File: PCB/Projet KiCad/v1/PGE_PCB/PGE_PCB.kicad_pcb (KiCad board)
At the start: 2 copper layers, 77 x 61.5 mm, 50 parts, among them CN2 Conn_01x02, J1 Conn_01x03, P1 USB_C_Plug_USB2.0, SW1 SW_Push, U1 STM32L476RGTx, U2 MCP73831T, U3 DS2438AZ+, U4 LD39050PU33R, U5 SiP32431DR3, Y1 ABS25-32.768KHZ-T

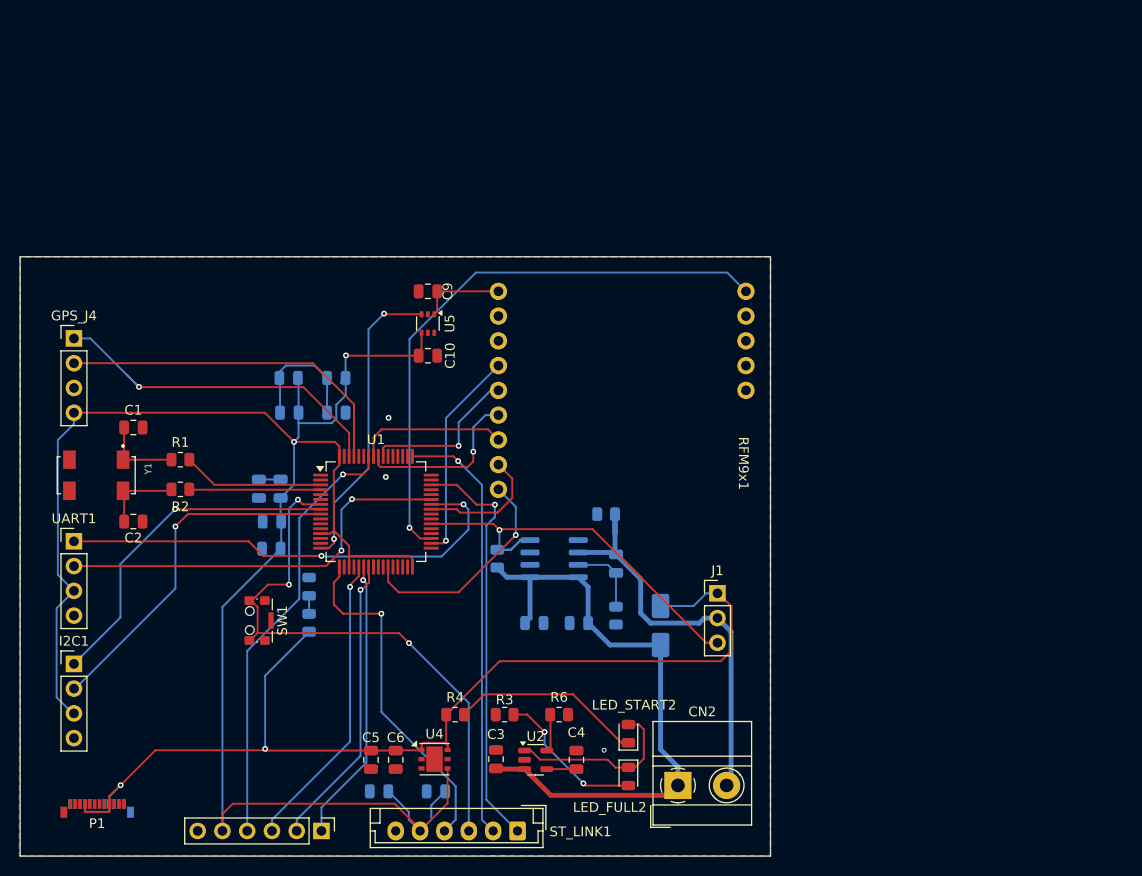
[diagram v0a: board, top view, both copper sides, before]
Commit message: Pcb VERSION GPS séparer
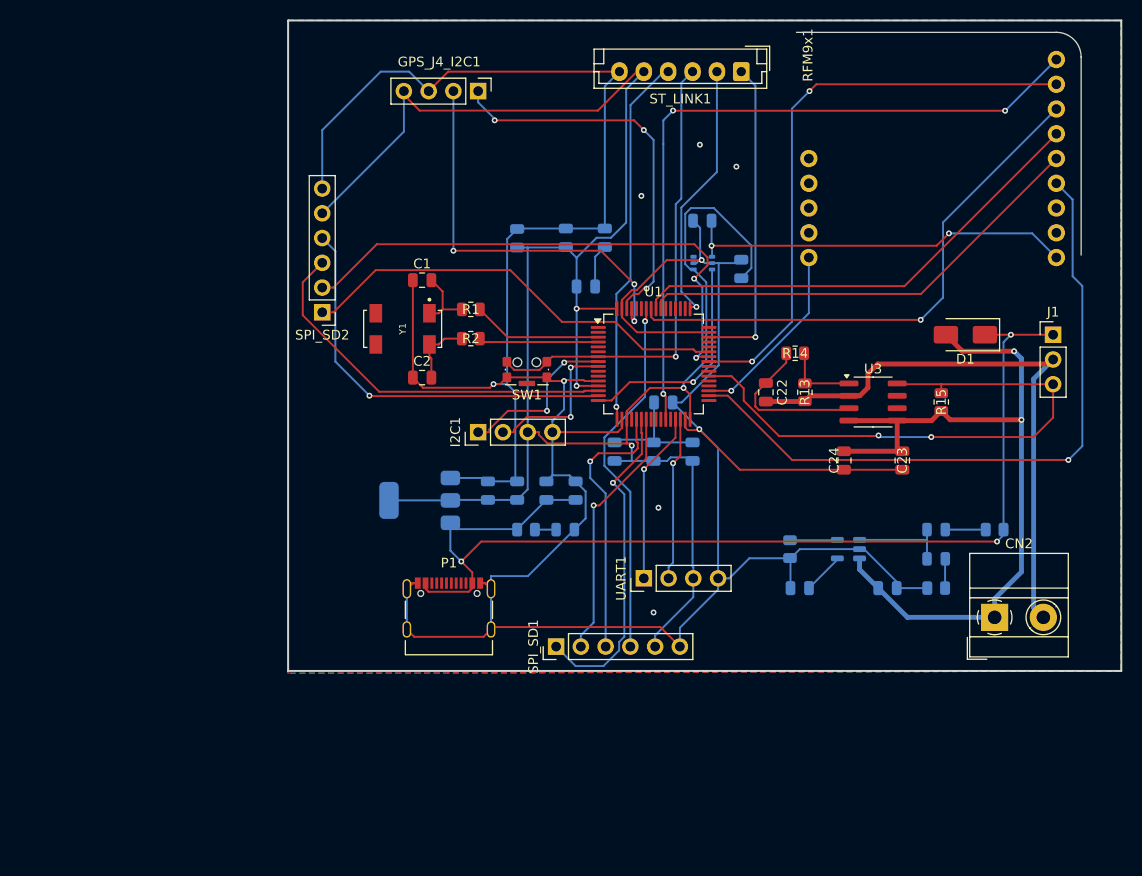
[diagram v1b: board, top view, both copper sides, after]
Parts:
- removed GPS_J4: Conn_01x04_Pin, Connector_PinHeader_2.54mm:PinHeader_1x04_P2.54mm_Vertical
- removed U4: LD39050PU33R, Package_DFN_QFN:DFN-6-1EP_3x3mm_P0.95mm_EP1.7x2.6mm
- added GPS_J4_I2C1: Conn_01x04_Pin, Connector_PinHeader_2.54mm:PinHeader_1x04_P2.54mm_Vertical, F.Cu at (138.0, 46.0)
- added SPI_SD2: Conn_01x06_Socket, Connector_PinHeader_2.54mm:PinHeader_1x06_P2.54mm_Vertical, F.Cu at (122.0, 68.7)
- added U6: LD1117S33TR_SOT223, Package_TO_SOT_SMD:SOT-223-3_TabPin2, B.Cu at (132.0, 88.0)
- C10, C3, C4, C5, C6, C9, LED_FULL2, LED_START2, R3, R4, R6, U2, U5: moved to B.Cu
- C22, C23, C24, D1, R13, R14, R15, U3: moved to F.Cu
- P1: footprint Connector_USB:USB_C_Plug_Molex_105444 -> Connector_USB:USB_C_Receptacle_Palconn_UTC16-G
- moved ST_LINK1 81.2 mm to (165.0, 44.0)
- moved UART1 58.6 mm to (155.0, 96.0), turned to 90 degrees
- moved R4 58.5 mm to (191.0, 91.0), turned to 0 degrees
- moved R15 48.3 mm to (185.5, 77.9)
- moved I2C1 47.8 mm to (138.0, 81.0), turned to 90 degrees
- moved R3 46.1 mm to (185.0, 97.0)
- moved C19 44.0 mm to (147.0, 61.0), turned to 90 degrees
- moved C18 43.9 mm to (151.0, 61.0), turned to 90 degrees
- moved C3 43.8 mm to (180.0, 97.0), turned to 180 degrees
- moved J1 43.5 mm to (197.0, 71.0)
- moved D1 43.2 mm to (188.0, 71.0), turned to 180 degrees
- moved C14 42.1 mm to (160.0, 83.0), turned to 90 degrees
- moved P1 41.3 mm to (135.0, 99.0)
- moved RFM9x1 39.1 mm to (184.0, 52.7), turned to 90 degrees
- moved U2 38.7 mm to (176.0, 93.0), turned to 180 degrees
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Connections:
- U1 pad 14: unconnected-(U1-PA0-Pad14) -> standby
- U1 pad 15: unconnected-(U1-PA1-Pad15) -> GPS_reset
- U1 pad 29: unconnected-(U1-PB10-Pad29) -> Tx_uart
- U1 pad 30: unconnected-(U1-PB11-Pad30) -> Rx_uart
- U1 pad 42: Tx_uart -> GPS_RX
- U1 pad 43: Rx_uart -> GPS_TX
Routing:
- net VREF-: track 0.00 -> 348.6 mm, vias 3 -> 9
- net GPS_RX: track 0.00 -> 54.8 mm, vias 0 -> 2
- net LoRa_RST: track 22.9 -> 73.7 mm, vias 1 -> 3
- net LORA_G0: track 21.8 -> 69.7 mm
- net LoRa_CS: track 13.1 -> 60.3 mm, vias 0 -> 2
- net GPS_TX: track 0.00 -> 44.9 mm
- net GPS_reset: track 0.00 -> 41.8 mm, vias 0 -> 1
- net LORA_G1: track 60.2 -> 19.3 mm
- net LoRa_MOSI: track 15.6 -> 56.0 mm, vias 0 -> 1
- net standby: track 0.00 -> 39.8 mm
- net VDD_LORA: track 8.77 -> 40.7 mm, vias 0 -> 2
- net LoRa_MISO: track 17.5 -> 49.1 mm, vias 1 -> 0
- net LoRa_SCK: track 16.6 -> 47.5 mm, vias 1 -> 0
- net Tx_uart: track 48.5 -> 17.7 mm, vias 2 -> 1
- net Rx_uart: track 42.0 -> 16.8 mm, vias 2 -> 1
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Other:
- board size 77 x 61.5 mm -> 85.5 x 66.8 mm
